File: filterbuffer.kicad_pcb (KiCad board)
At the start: 2 copper layers, 143 x 45 mm, 27 parts, among them J1 Conn_01x02, J10 Conn_01x02, J11 Conn_01x02, J12 Conn_01x02, J13 Conn_01x02, J14 Conn_01x02, J15 Conn_01x02, J16 Conn_01x02, J2 Conn_01x02, J3 Conn_01x02, J4 Conn_01x02, J5 Conn_01x02, J6 Conn_01x02, J7 Conn_01x02, J8 Conn_01x02, J9 Conn_01x02

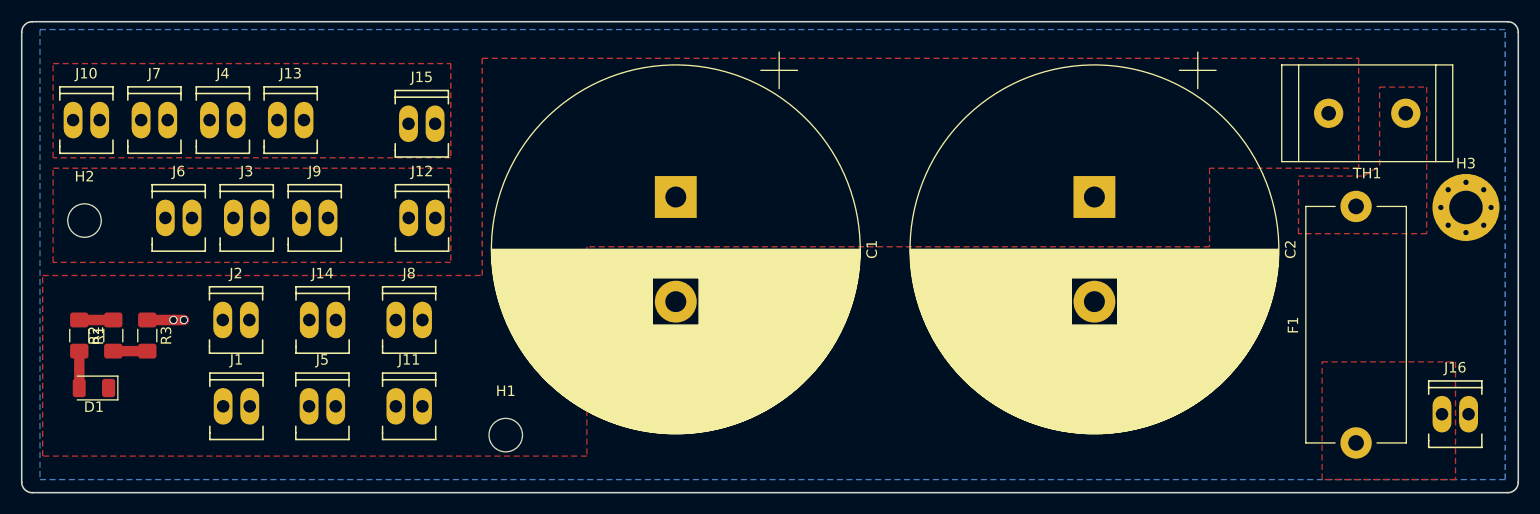
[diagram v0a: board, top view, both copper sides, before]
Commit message: layout redesign
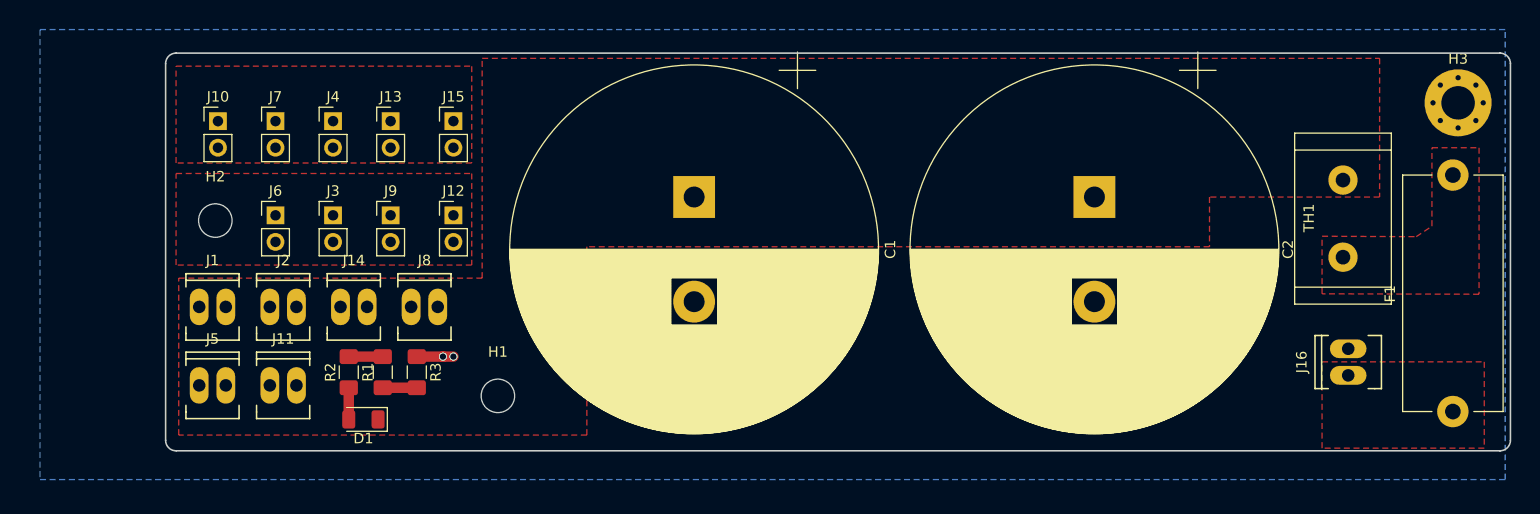
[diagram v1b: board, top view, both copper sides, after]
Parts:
- J10, J12, J13, J15, J3, J4, J6, J7, J9: footprint Sockets_MOLEX_KK-System:Socket_MOLEX-KK-RM2-54mm_Lock_2pin_straight -> Connector_PinHeader_2.54mm:PinHeader_1x02_P2.54mm_Vertical
- moved R1 26.0 mm to (74.7, 129.9)
- moved R2 26.0 mm to (78.0, 129.9)
- moved R3 26.0 mm to (81.2, 129.9)
- moved D1 25.9 mm to (76.1, 134.4)
- moved TH1 15.0 mm to (169.7, 119.0), turned to 90 degrees
- moved J10 12.6 mm to (62.2, 106.0)
- moved H2 12.5 mm to (62.0, 115.5)
- moved J11 12.2 mm to (68.4, 131.2)
- moved J7 11.6 mm to (67.7, 106.0)
- moved J16 11.4 mm to (170.2, 129.0), turned to 90 degrees
- moved J5 10.7 mm to (61.7, 131.2)
- moved J4 10.5 mm to (73.2, 106.0)
- moved H3 10.0 mm to (180.7, 104.2)
- moved J1 9.77 mm to (61.7, 123.7)
- moved F1 9.72 mm to (180.2, 133.7)
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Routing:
- net Net-(D1-Pad2): track 3.52 -> 3.02 mm
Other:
- board size 143 x 45 mm -> 128.5 x 38 mm
